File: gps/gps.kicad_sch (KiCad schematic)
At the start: 23 parts, among them J1 I2C/BATT_H, J2 I2C/BATT_S, J3 USB_pads, J4 BATT, J5 ESP, SW2 MSN22AFW01, U1 NEO-M9N, U2 TPS613222ADBVR

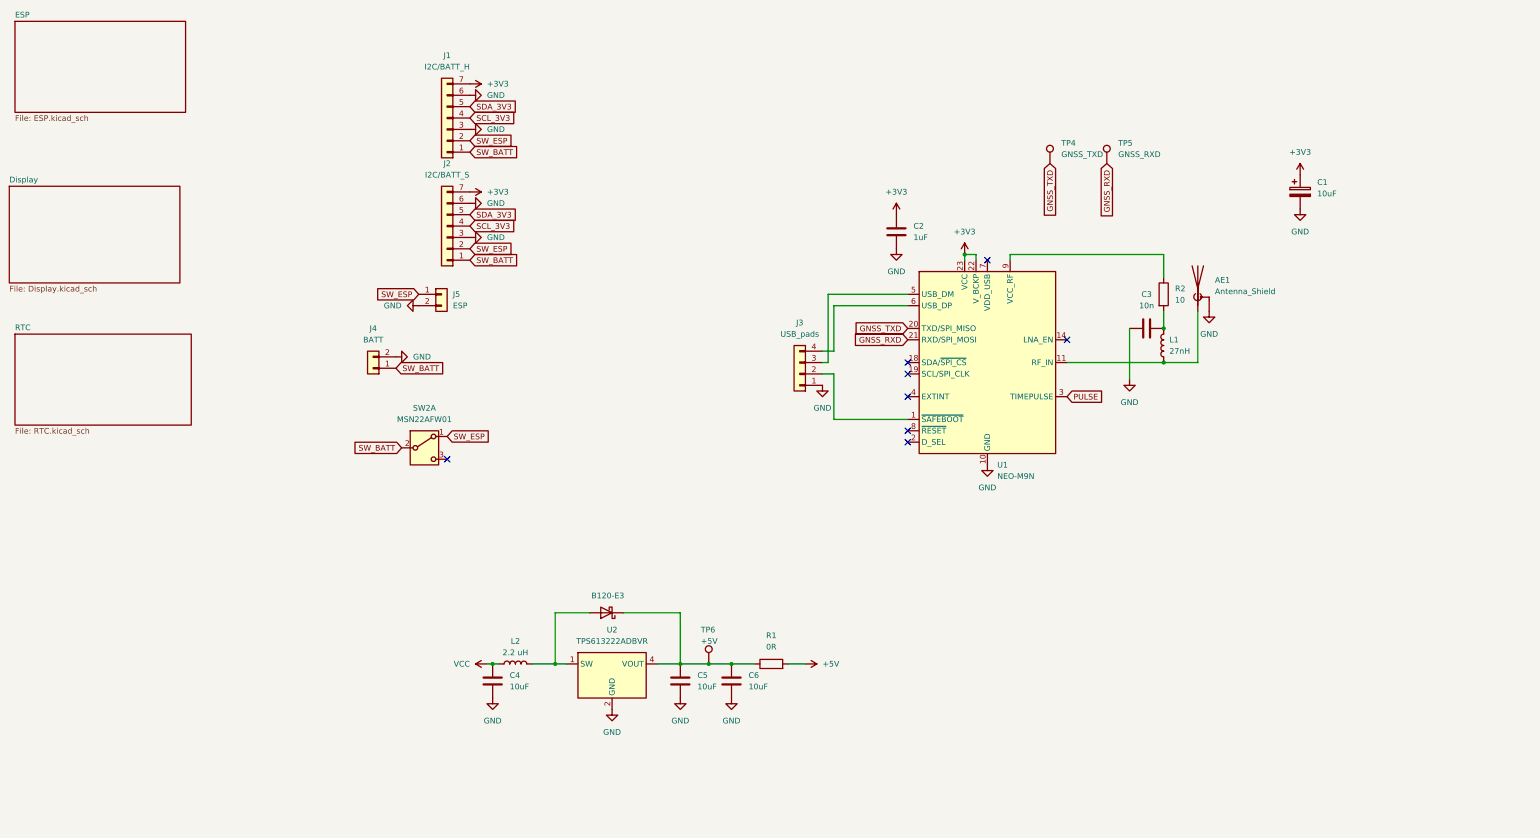
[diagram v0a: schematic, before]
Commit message: cleaned schematic
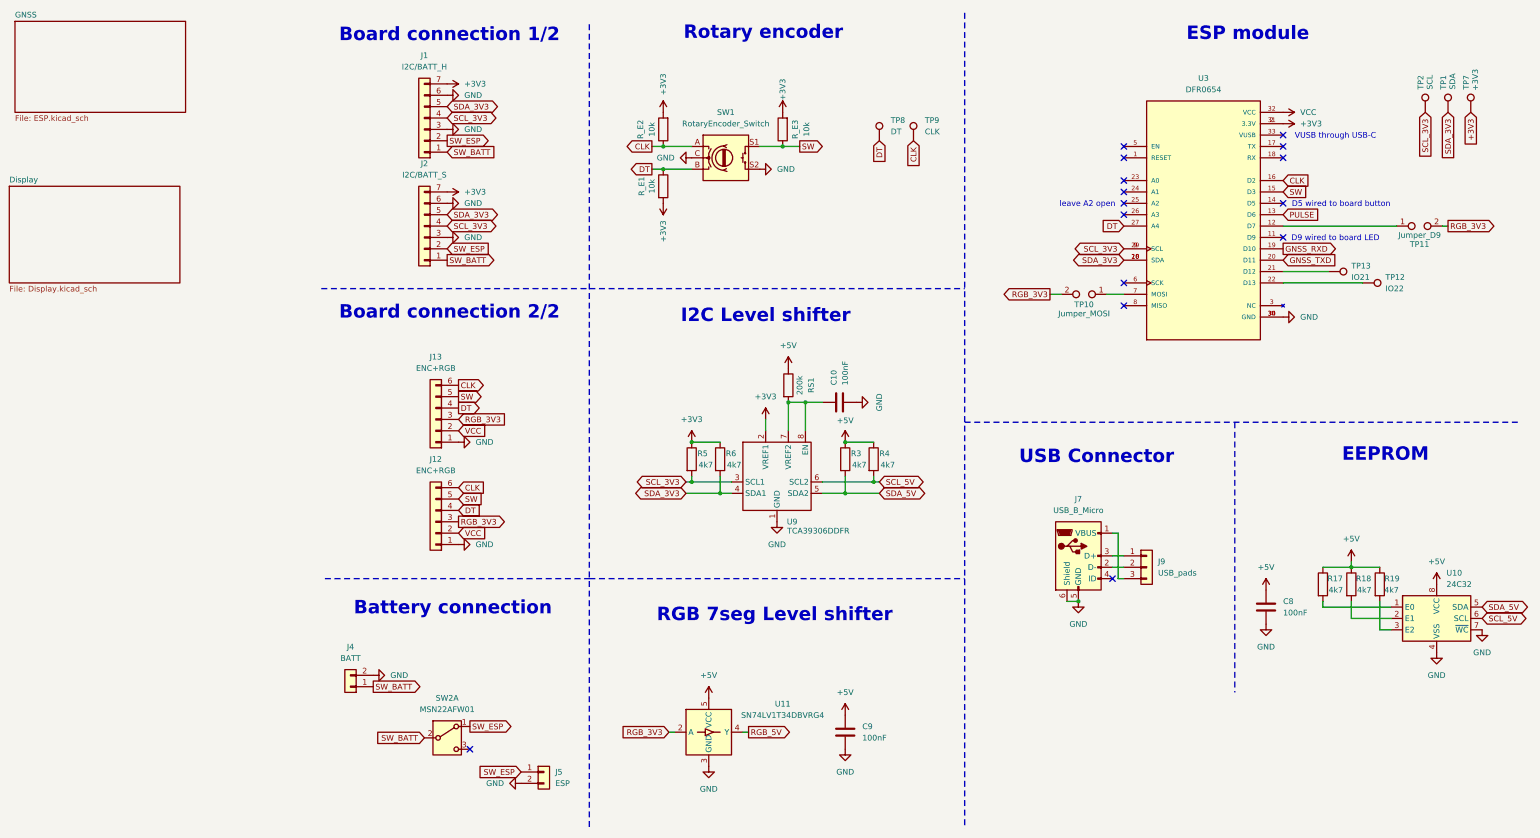
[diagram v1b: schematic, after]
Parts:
- removed AE1: Antenna_Shield, w_conn_rf:lemo_epb00250ntn, symbol Device:Antenna_Shield
- removed C1: 10uF, Capacitor_Tantalum_SMD:CP_EIA-3528-15_AVX-H_Pad1.50x2.35mm_HandSolder, symbol Device:C_Polarized
- removed C2: 1uF, Capacitor_SMD:C_0603_1608Metric_Pad1.08x0.95mm_HandSolder, symbol Device:C
- removed C3: 10n, Capacitor_SMD:C_0805_2012Metric_Pad1.18x1.45mm_HandSolder, symbol Device:C
- removed C4, C5, C6: 10uF, Capacitor_SMD:C_0603_1608Metric_Pad1.08x0.95mm_HandSolder, symbol Device:C
- removed D2: B120-E3, Diode_SMD:D_SMA, symbol Diode:B120-E3
- removed J3: USB_pads, Connector_PinHeader_2.54mm:PinHeader_1x04_P2.54mm_Vertical, symbol Connector_Generic:Conn_01x04
- removed L1: 27nH, Inductor_SMD:L_0402_1005Metric_Pad0.77x0.64mm_HandSolder, symbol Device:L
- removed L2: 2.2 uH, Inductor_SMD:L_1008_2520Metric_Pad1.43x2.20mm_HandSolder, symbol Device:L
- removed R1: 0R, Resistor_SMD:R_0805_2012Metric_Pad1.20x1.40mm_HandSolder, symbol Device:R
- removed R2: 10, Resistor_SMD:R_1206_3216Metric_Pad1.30x1.75mm_HandSolder, symbol Device:R
- removed TP4: GNSS_TXD, TestPoint:TestPoint_Loop_D1.80mm_Drill1.0mm_Beaded, symbol Connector:TestPoint
- removed TP5: GNSS_RXD, TestPoint:TestPoint_Loop_D1.80mm_Drill1.0mm_Beaded, symbol Connector:TestPoint
- removed TP6: +5V, TestPoint:TestPoint_Loop_D1.80mm_Drill1.0mm_Beaded, symbol Connector:TestPoint
- removed U1: NEO-M9N, RF_GPS:ublox_NEO, symbol RF_GPS:NEO-M8N
- removed U2: TPS613222ADBVR, Package_TO_SOT_SMD:SOT-23-5, symbol Regulator_Switching:TPS613226ADBV
- added C10, C8, C9: 100nF, Capacitor_SMD:C_0805_2012Metric_Pad1.18x1.45mm_HandSolder, symbol Device:C
- added J12: ENC+RGB, Connector_PinSocket_2.54mm:PinSocket_1x06_P2.54mm_Vertical, symbol Connector_Generic:Conn_01x06
- added J13: ENC+RGB, Connector_PinHeader_2.54mm:PinHeader_1x06_P2.54mm_Vertical, symbol Connector_Generic:Conn_01x06
- added J7: USB_B_Micro, KiCad:USB3145301A, symbol Connector:USB_B_Micro
- added J9: USB_pads, Connector_PinSocket_2.54mm:PinSocket_1x03_P2.54mm_Vertical, symbol Connector_Generic:Conn_01x03
- added R17, R18, R19, R3, R4, R5, R6: 4k7, Resistor_SMD:R_0805_2012Metric_Pad1.20x1.40mm_HandSolder, symbol Device:R
- added RS1: 200k, Resistor_SMD:R_0805_2012Metric_Pad1.20x1.40mm_HandSolder, symbol Device:R
- added R_E1, R_E2, R_E3: 10k, Resistor_SMD:R_0805_2012Metric_Pad1.20x1.40mm_HandSolder, symbol Device:R
- added SW1: RotaryEncoder_Switch, Rotary_Encoder:RotaryEncoder_20mm_WO_mount_holes, symbol Device:RotaryEncoder_Switch
- added TP1: SDA, TestPoint:TestPoint_Loop_D1.80mm_Drill1.0mm_Beaded, symbol Connector:TestPoint
- added TP10: Jumper_MOSI, Resistor_SMD:R_0805_2012Metric_Pad1.20x1.40mm_HandSolder, symbol Connector:TestPoint_2Pole
- added TP11: Jumper_D9, Resistor_SMD:R_0805_2012Metric_Pad1.20x1.40mm_HandSolder, symbol Connector:TestPoint_2Pole
- added TP12: IO22, TestPoint:TestPoint_Loop_D1.80mm_Drill1.0mm_Beaded, symbol Connector:TestPoint
- added TP13: IO21, TestPoint:TestPoint_Loop_D1.80mm_Drill1.0mm_Beaded, symbol Connector:TestPoint
- added TP2: SCL, TestPoint:TestPoint_Loop_D1.80mm_Drill1.0mm_Beaded, symbol Connector:TestPoint
- added TP7: +3V3, TestPoint:TestPoint_Loop_D1.80mm_Drill1.0mm_Beaded, symbol Connector:TestPoint
- added TP8: DT, TestPoint:TestPoint_Loop_D1.80mm_Drill1.0mm_Beaded, symbol Connector:TestPoint
- added TP9: CLK, TestPoint:TestPoint_Loop_D1.80mm_Drill1.0mm_Beaded, symbol Connector:TestPoint
- added U10: 24C32, Package_SO:SOIC-8_3.9x4.9mm_P1.27mm, symbol Memory_EEPROM:M24C01-FMN
- added U11: SN74LV1T34DBVRG4, Package_TO_SOT_SMD:SOT-23-5, symbol Logic_LevelTranslator:SN74LV1T34DBV
- added U3: DFR0654, DFR0654:DFR0654_2, symbol DFR0654:DFR0654
- added U9: TCA39306DDFR, Package_TO_SOT_SMD:SOT-23-8, symbol shifter:TCA39306DCURQ1
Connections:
- net +3V3: now also R5.1, R6.1, R_E1.2, R_E2.2, R_E3.2, TP7.1, U3.2 (3.3V), U3.31 (3.3V), U9.2 (VREF1)
- net +5V: now also C8.2, C9.2, R17.1, R18.1, R19.1, R3.1, R4.1, RS1.1, U10.8 (VCC), U11.5 (VCC)
- net GND: now also C10.1, C8.1, C9.1, J12.1 (Pin_1), J13.1 (Pin_1), J7.5 (GND), J7.6 (Shield), SW1.C, SW1.S2, U10.4 (VSS), U10.7 (~{WC}), U11.3 (GND), U3.30 (GND), U3.34 (GND), U3.4 (GND), U9.1 (GND)
- net GNSS_RXD: now also U3.19 (D10)
- net GNSS_TXD: now also U3.20 (D11)
- net PULSE: now also U3.13 (D6)
- net SCL_3V3: now also R5.2, TP2.1, U3.29 (SCL), U3.9 (SCL), U9.3 (SCL1)
- net SDA_3V3: now also R6.2, TP1.1, U3.10 (SDA), U3.28 (SDA), U9.4 (SDA1)
- net VCC: now also J12.2 (Pin_2), J13.2 (Pin_2), U3.32 (VCC)
- new net: TP11.1, U3.12 (D7)
- new net: TP13.1, U3.21 (D12)
- new net: TP12.1, U3.22 (D13)
- new net: TP10.1, U3.7 (MOSI)
- new net: R17.2, U10.1 (E0)
- new net: R18.2, U10.2 (E1)
- new net: R19.2, U10.3 (E2)
- new net: C10.2, RS1.2, U9.7 (VREF2), U9.8 (EN)
- new net: J7.1 (VBUS), J9.3 (Pin_3)
- new net: J7.2 (D-), J9.2 (Pin_2)
- new net: J7.3 (D+), J9.1 (Pin_1)
- new net CLK: J12.6 (Pin_6), J13.6 (Pin_6), R_E2.1, SW1.A, TP9.1, U3.16 (D2)
- new net DT: J12.4 (Pin_4), J13.4 (Pin_4), R_E1.1, SW1.B, TP8.1, U3.27 (A4)
- new net RGB_3V3: J12.3 (Pin_3), J13.3 (Pin_3), TP10.2, TP11.2, U11.2 (A)
- new net RGB_5V: U11.4 (Y)
- new net SCL_5V: R4.2, U10.6 (SCL), U9.6 (SCL2)
- new net SDA_5V: R3.2, U10.5 (SDA), U9.5 (SDA2)
- new net SW: J12.5 (Pin_5), J13.5 (Pin_5), R_E3.1, SW1.S1, U3.15 (D3)
- no-connect marks 8 -> 15
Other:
- sheet ESP renamed GNSS
- removed sheet RTC
- note added: "Battery connection"
- note added: "Board connection 1/2"
- note added: "Board connection 2/2"
- note added: "D5 wired to board button"
- note added: "D9 wired to board LED"
- note added: "EEPROM"
- note added: "ESP module"
- note added: "I2C Level shifter"
- note added: "RGB 7seg Level shifter"
- note added: "Rotary encoder"
- note added: "USB Connector"
- note added: "VUSB through USB-C"
- note added: "leave A2 open"
- moved on the sheet: J1, J2, J4, J5, SW2A
